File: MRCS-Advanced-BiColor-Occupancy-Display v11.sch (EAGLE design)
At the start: 4 parts

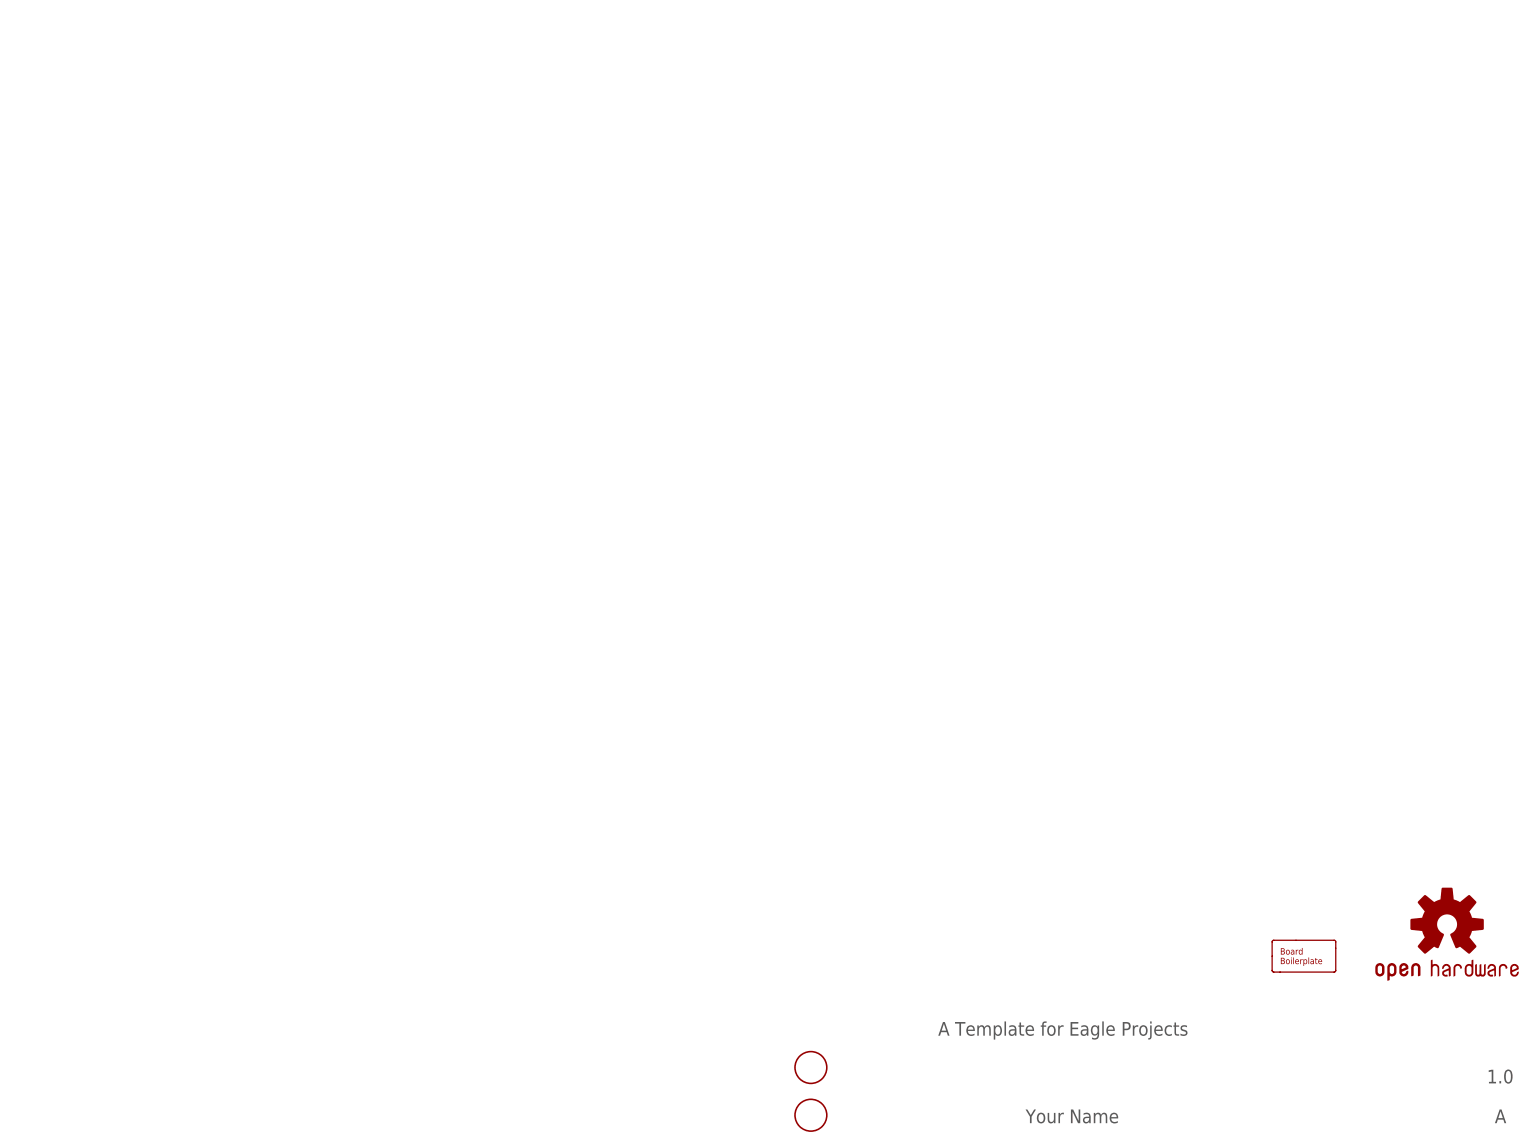
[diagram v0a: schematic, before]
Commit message: imported work files into GitHub
moving work files around to clean up documentation
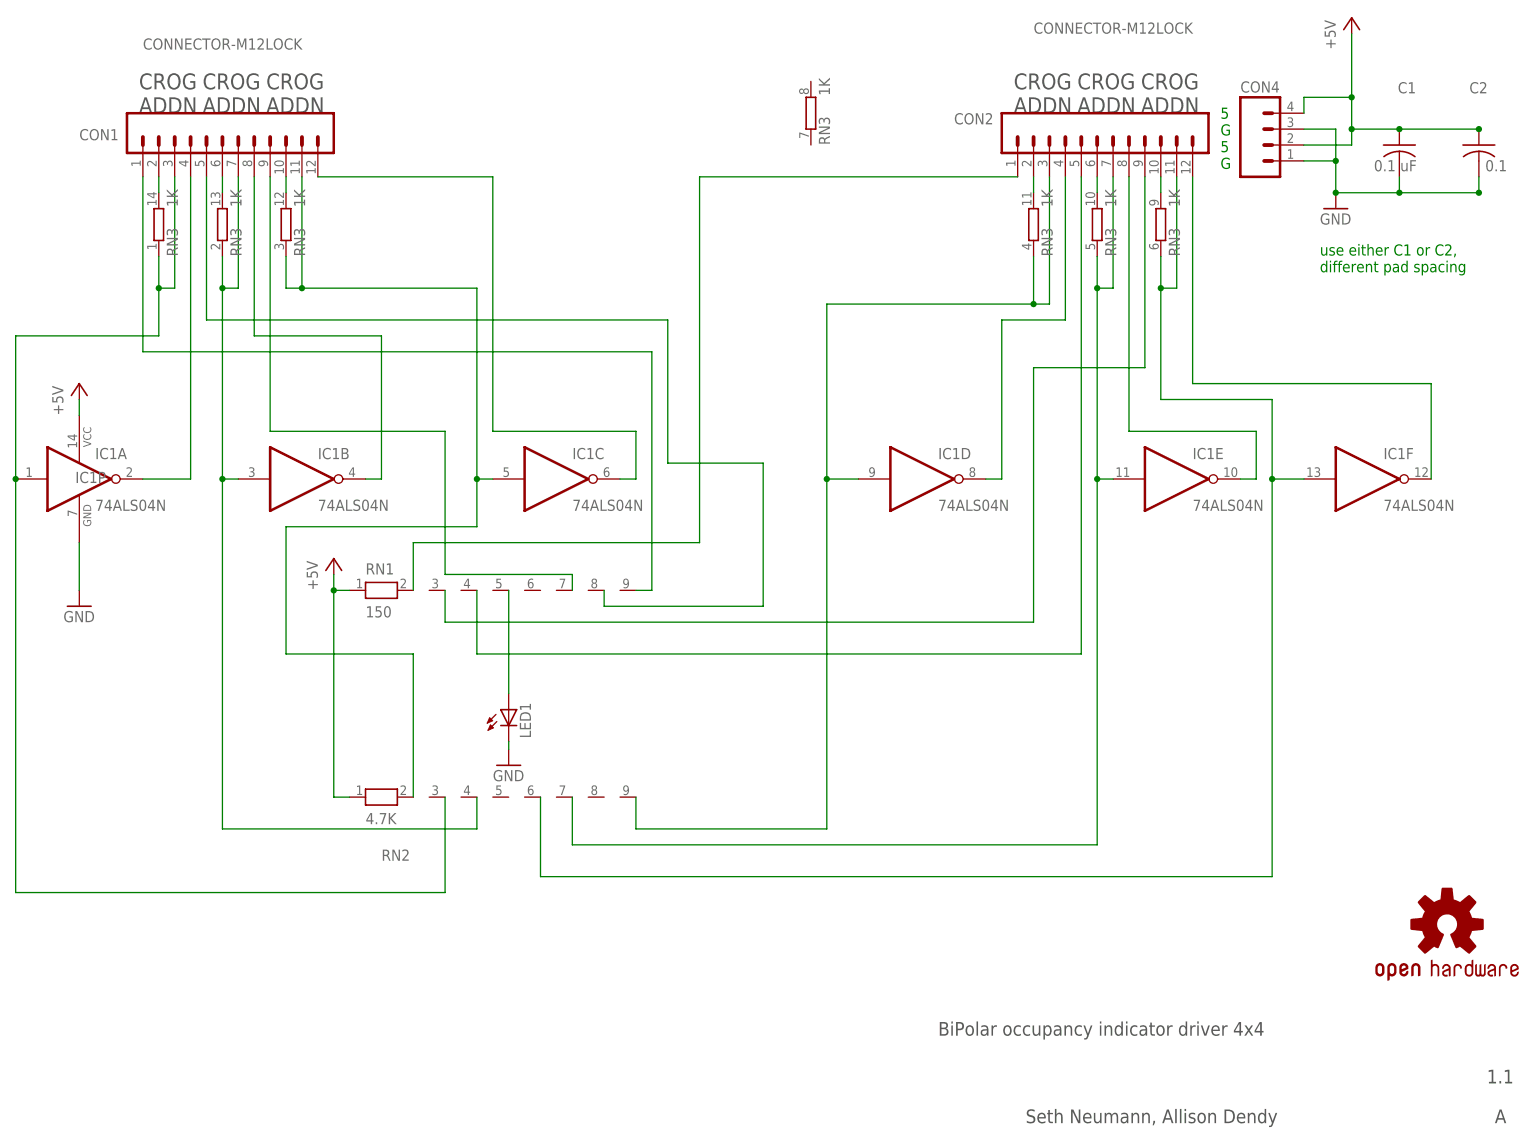
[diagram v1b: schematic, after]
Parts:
- removed BOARD1: BOARD80X100, SPCoast:BOARD80X100
- removed FID1, FID2: FIDUCIAL, SPCoast:FIDUCIAL
- added C1: 0.1 uF, SPCoast:CAPPTH2
- added C2: 0.1, SPCoast:CAPPTH1
- added CON1, CON2: CONNECTOR-M12LOCK, SPCoast:CONNECTOR-M12LOCK
- added CON4: (no value), SPCoast:CONNECTOR-M04SCREW
- added IC1: 74ALS04N, 74xx-us:74ALS04N
- added LED1: (no value), SPCoast:LEDLED3MM
- added RN1: 150, resistor-net:RN08
- added RN2: 4.7K, resistor-net:RN08
- added RN3: 1K, resistor-dil:7R-P
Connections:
- new net GND: C1.2, C2.2, CON4.1, CON4.3, IC1P.GND, LED1.C
- new net N$1: CON1.2, RN3A.2
- new net N$10: CON1.9, RN1.7
- new net N$11: CON2.8, IC1E.O
- new net N$12: CON2.12, IC1F.O
- new net N$13: CON2.4, IC1D.O
- new net N$14: CON2.1, RN1.2
- new net N$15: CON2.5, RN1.4
- new net N$16: CON1.3, IC1A.I, RN2.3, RN3A.1
- new net N$17: LED1.A, RN1.5
- new net N$18: CON2.7, IC1E.I, RN2.7, RN3E.1
- new net N$19: CON2.9, RN1.3
- new net N$2: CON1.11, IC1C.I, RN2.2, RN3C.1
- new net N$20: CON2.11, IC1F.I, RN2.6, RN3F.1
- new net N$21: CON1.6, RN3B.2
- new net N$22: CON1.10, RN3C.2
- new net N$23: CON2.2, RN3D.2
- new net N$24: CON2.6, RN3E.2
- new net N$25: CON2.10, RN3F.2
- new net N$3: CON1.1, RN1.9
- new net N$4: CON1.4, IC1A.O
- new net N$5: CON1.7, IC1B.I, RN2.4, RN3B.1
- new net N$6: CON1.12, IC1C.O
- new net N$7: CON1.8, IC1B.O
- new net N$8: CON1.5, RN1.8
- new net N$9: CON2.3, IC1D.I, RN2.9, RN3D.1
- new net VCC: C1.1, C2.1, CON4.2, CON4.4, IC1P.VCC, RN1.1, RN2.1
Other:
- note added: "1.1"
- note added: "5 G 5 G"
- note added: "BiPolar occupancy indicator driver 4x4"
- note added: "CROG ADDN"
- note added: "Seth Neumann, Allison Dendy"
- note added: "use either C1 or C2, different pad spacing"
- note removed: "1.0"
- note removed: "A Template for Eagle Projects"
- note removed: "Your Name"
